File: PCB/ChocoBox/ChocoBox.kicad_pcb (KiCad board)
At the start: 2 copper layers, 8 parts, among them J1 DTH22_01, J2 DTH22_02, J3 DS3231, J4 LCD2004A, J5 microSD, J6 Humidificador, J7 WTR, U1 ESP32-DEVKIT-V1

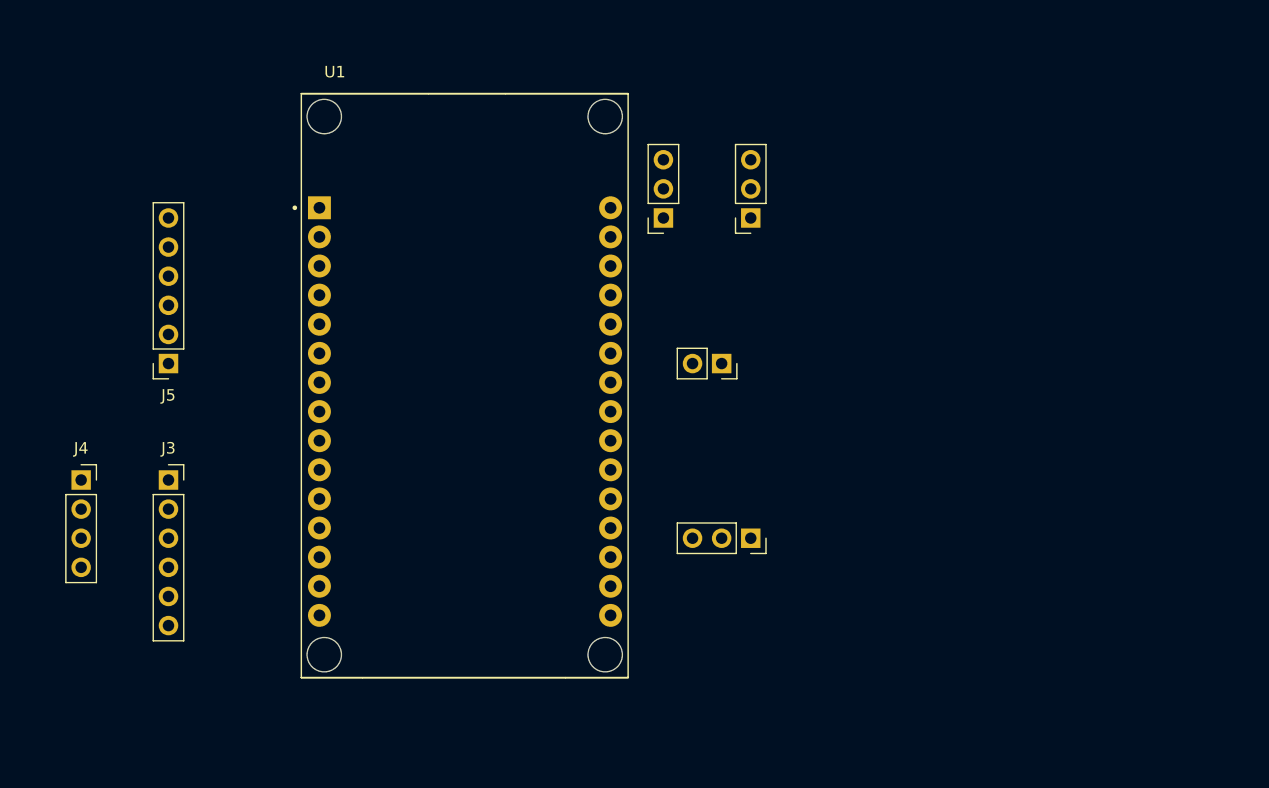
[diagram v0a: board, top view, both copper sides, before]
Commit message: PCB V1 Terminada
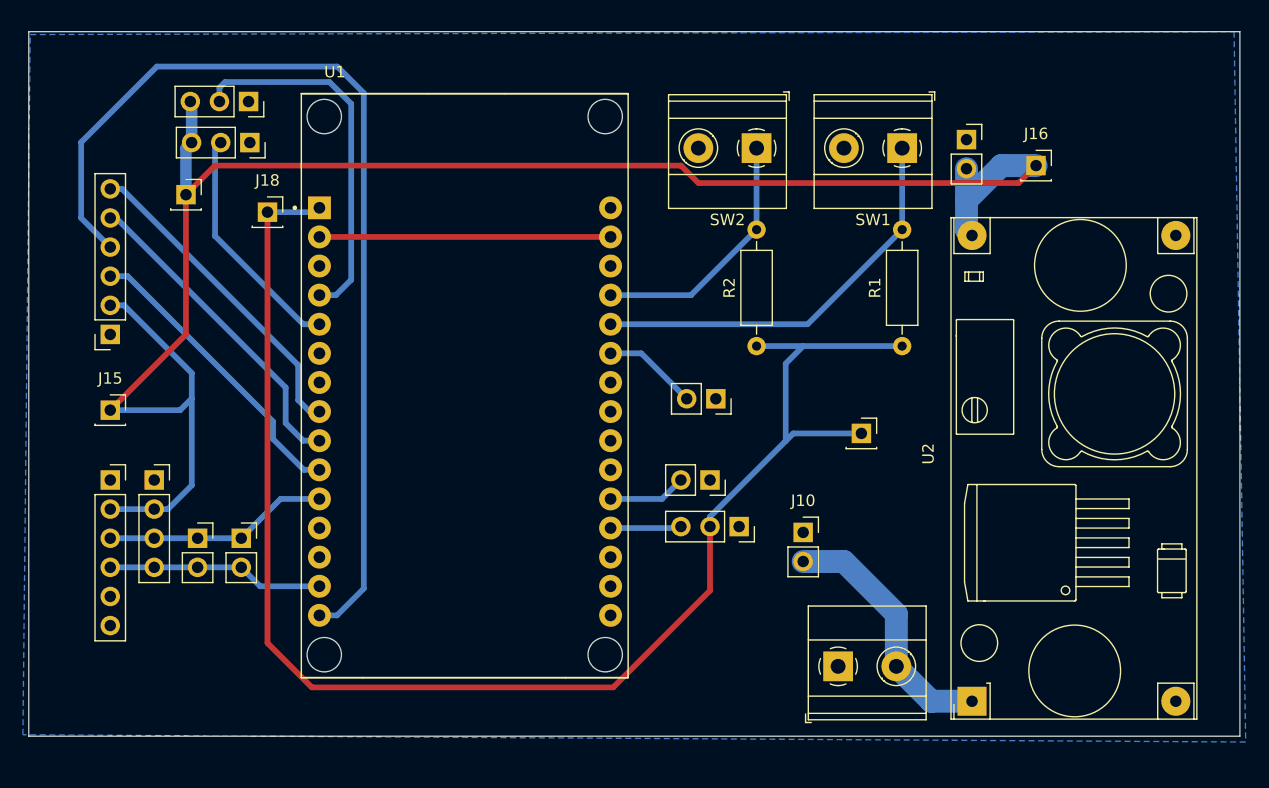
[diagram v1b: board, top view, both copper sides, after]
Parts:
- added J10: Vout-12V, Connector_PinSocket_2.54mm:PinSocket_1x02_P2.54mm_Vertical, F.Cu at (129.0, 80.8)
- added J11: Conn_01x01, Connector_PinSocket_2.54mm:PinSocket_1x01_P2.54mm_Vertical, F.Cu at (75.2, 51.3)
- added J12: I2C, Connector_PinSocket_2.54mm:PinSocket_1x02_P2.54mm_Vertical, F.Cu at (76.2, 81.3)
- added J13: I2C, Connector_PinSocket_2.54mm:PinSocket_1x02_P2.54mm_Vertical, F.Cu at (80.0, 81.3)
- added J14: Vout-5V, Connector_PinSocket_2.54mm:PinSocket_1x02_P2.54mm_Vertical, F.Cu at (143.3, 46.5)
- added J15: Conn_01x01, Connector_PinSocket_2.54mm:PinSocket_1x01_P2.54mm_Vertical, F.Cu at (68.6, 70.1)
- added J16: Conn_01x01, Connector_PinSocket_2.54mm:PinSocket_1x01_P2.54mm_Vertical, F.Cu at (149.4, 48.8)
- added J17: Conn_01x01, Connector_PinSocket_2.54mm:PinSocket_1x01_P2.54mm_Vertical, F.Cu at (134.1, 72.1)
- added J18: Conn_01x01, Connector_PinSocket_2.54mm:PinSocket_1x01_P2.54mm_Vertical, F.Cu at (82.3, 52.8)
- added J8: Vin, TerminalBlock_Phoenix:TerminalBlock_Phoenix_MKDS-1,5-2-5.08_1x02_P5.08mm_Horizontal, F.Cu at (132.1, 92.5)
- added J9: Calentador, Connector_PinSocket_2.54mm:PinSocket_1x02_P2.54mm_Vertical, F.Cu at (120.9, 76.2)
- added R1: 10K, Resistor_THT:R_Axial_DIN0207_L6.3mm_D2.5mm_P10.16mm_Horizontal, F.Cu at (137.7, 64.5)
- added R2: 10K, Resistor_THT:R_Axial_DIN0207_L6.3mm_D2.5mm_P10.16mm_Horizontal, F.Cu at (125.0, 64.5)
- added SW1: BTN1, TerminalBlock_Phoenix:TerminalBlock_Phoenix_MKDS-1,5-2-5.08_1x02_P5.08mm_Horizontal, F.Cu at (137.7, 47.2)
- added SW2: BTN2, TerminalBlock_Phoenix:TerminalBlock_Phoenix_MKDS-1,5-2-5.08_1x02_P5.08mm_Horizontal, F.Cu at (125.0, 47.2)
- added U2: DCDC_StepDown_LM2596, Custom:YAAJ_DCDC_StepDown_LM2596, F.Cu at (143.8, 95.5)
- J7: value WTR -> WaterLevel
- moved J2 45.0 mm to (80.6, 43.2), turned to -90 degrees
- moved J1 36.7 mm to (80.8, 46.8), turned to -90 degrees
- moved J4 6.38 mm to (72.4, 76.2)
- moved J5 5.68 mm to (68.6, 63.5)
- moved J3 5.08 mm to (68.6, 76.2)
- moved J6 3.11 mm to (121.4, 69.1)
- moved J7 1.44 mm to (123.4, 80.3)
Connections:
- U1 pad 20: unconnected-(U1-D35-Pad20) -> GPIO_35
- U1 pad 26: unconnected-(U1-D14-Pad26) -> BTN1
- U1 pad 27: unconnected-(U1-D12-Pad27) -> BTN2
- U1 pad 30: +5V -> Vdrive
- U1 pad 6: unconnected-(U1-RX2-Pad6) -> RX2
- U1 pad 7: unconnected-(U1-TX2-Pad7) -> TX2
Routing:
- net +5V: track 0.00 -> 154.4 mm
- net +3.3V: track 0.00 -> 130.3 mm
- net MOSI: track 0.00 -> 86.6 mm
- net BTN1: track 0.00 -> 36.0 mm
- net GPIO_02: track 0.00 -> 32.4 mm
- net CS: track 0.00 -> 28.1 mm
- net SCK: track 0.00 -> 27.6 mm
- net MISO: track 0.00 -> 26.1 mm
- net GND: track 0.00 -> 25.4 mm
- net +12V: track 0.00 -> 22.5 mm
- net BTN2: track 0.00 -> 22.2 mm
- net GPIO_04: track 0.00 -> 20.7 mm
- net GPIO_SDA: track 0.00 -> 19.7 mm
- net GPIO_SCL: track 0.00 -> 18.9 mm
- net GPIO_27: track 0.00 -> 8.28 mm
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- added copper zone on B.Cu, net GND
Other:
- board outline added: 105.7 x 61.5 mm

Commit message: PCB terminada
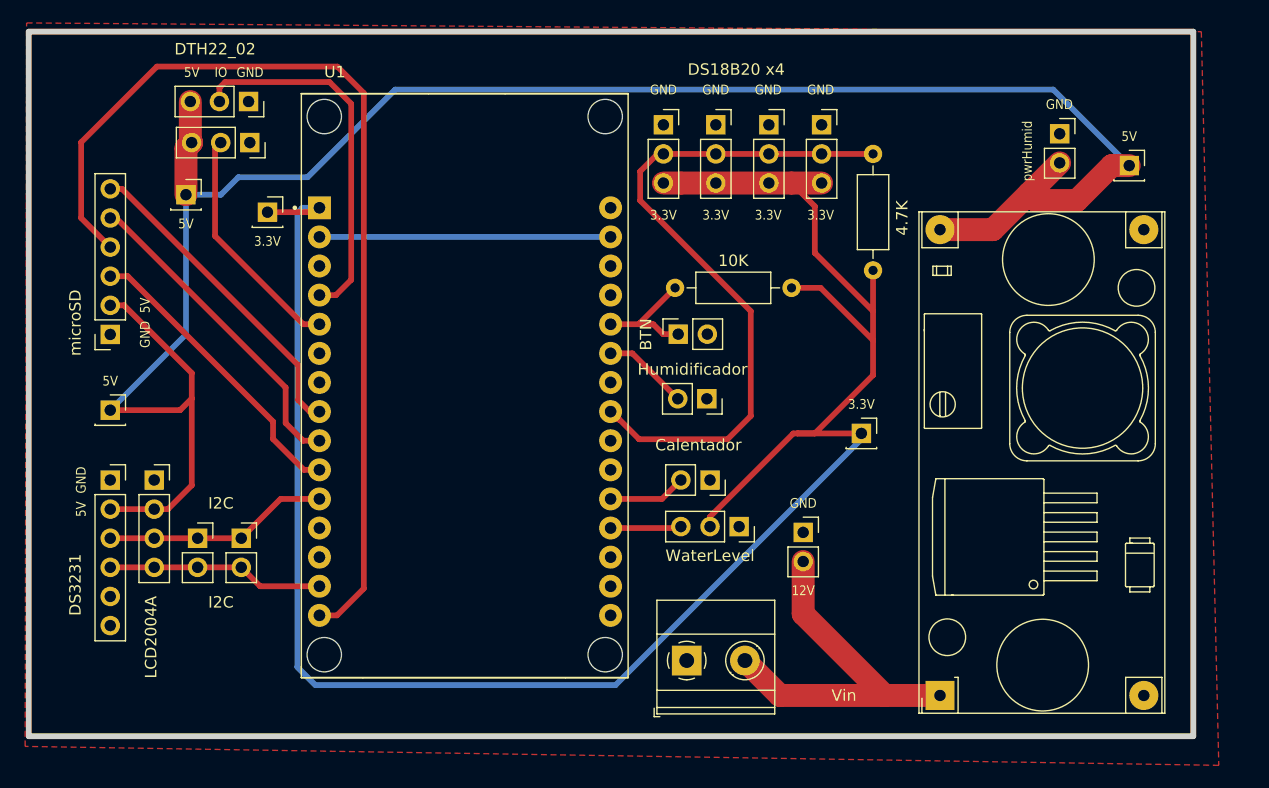
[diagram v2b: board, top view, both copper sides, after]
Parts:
- removed R2: 10K, Resistor_THT:R_Axial_DIN0207_L6.3mm_D2.5mm_P10.16mm_Horizontal
- removed SW2: BTN2, TerminalBlock_Phoenix:TerminalBlock_Phoenix_MKDS-1,5-2-5.08_1x02_P5.08mm_Horizontal
- added J19: DS18B20-A, Connector_PinSocket_2.54mm:PinSocket_1x03_P2.54mm_Vertical, F.Cu at (116.8, 45.2)
- added J20: DS18B20-B, Connector_PinSocket_2.54mm:PinSocket_1x03_P2.54mm_Vertical, F.Cu at (121.4, 45.2)
- added J21: DS18B20-C, Connector_PinSocket_2.54mm:PinSocket_1x03_P2.54mm_Vertical, F.Cu at (126.0, 45.2)
- added J22: DS18B20-D, Connector_PinSocket_2.54mm:PinSocket_1x03_P2.54mm_Vertical, F.Cu at (130.6, 45.2)
- added R3: 4.7K, Resistor_THT:R_Axial_DIN0207_L6.3mm_D2.5mm_P10.16mm_Horizontal, F.Cu at (135.1, 47.8)
- J14: value Vout-5V -> Vout-5V-Humidificador
- SW1: footprint TerminalBlock_Phoenix:TerminalBlock_Phoenix_MKDS-1,5-2-5.08_1x02_P5.08mm_Horizontal -> Connector_PinSocket_2.54mm:PinSocket_1x02_P2.54mm_Vertical
- moved SW1 25.4 mm to (118.1, 63.5), turned to 90 degrees
- moved J8 13.2 mm to (118.9, 91.9)
- moved R1 10.9 mm to (128.0, 59.4), turned to 180 degrees
- moved J14 8.14 mm to (151.4, 46.0)
- moved J16 8.13 mm to (157.5, 48.8)
- moved U2 2.84 mm to (141.0, 95.0)
- moved J6 0.78 mm to (120.6, 69.1)
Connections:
- U1 pad 23: unconnected-(U1-D25-Pad23) -> OneWire
- U1 pad 27: BTN2 -> unconnected-(U1-D12-Pad27)
- U1 pad 6: RX2 -> unconnected-(U1-RX2-Pad6)
- U1 pad 7: TX2 -> unconnected-(U1-TX2-Pad7)
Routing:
- net OneWire: track 0.00 -> 59.8 mm
- net +3.3V: track 130.3 -> 176.5 mm
- net BTN1: track 36.0 -> 10.7 mm
- net +5V: track 154.4 -> 176.7 mm
- net BTN2: track 22.2 -> 0.00 mm
- net +12V: track 22.5 -> 32.9 mm
- net GPIO_27: track 8.28 -> 7.50 mm
- added copper zone on F.Cu, net GND
- removed copper zone on B.Cu, net GND
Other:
- board size 105.7 x 61.5 mm -> 101.6 x 61.5 mm
- board text added: "12V"
- board text added: "3.3V"
- board text added: "5V"
- board text added: "BTN"
- board text added: "DS18B20 x4"
- board text added: "GND"
- board text added: "IO"
- board text added: "pwrHumid"
